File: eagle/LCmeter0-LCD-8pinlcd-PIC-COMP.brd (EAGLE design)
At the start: 58.4 x 50.8 mm, 34 parts, among them IC1 PIC16F876A-X/SP, J1 HD44780-4BIT-8PIN, J2 PIC-UART, J3 PIC-ICSP, K2 DS2Y, Q1 20MHz, T1 BC547CBE-A, X1 FREQ, X2 L/C

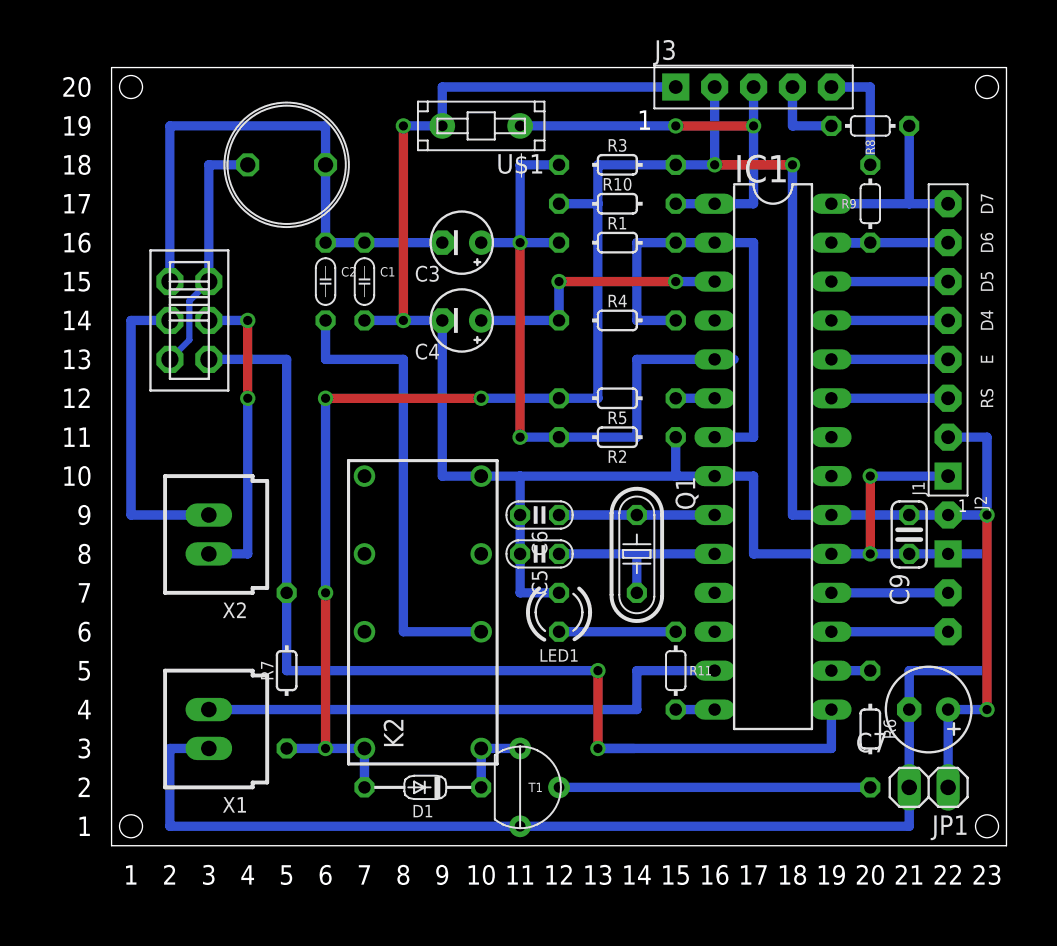
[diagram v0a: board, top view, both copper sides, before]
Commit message: ...
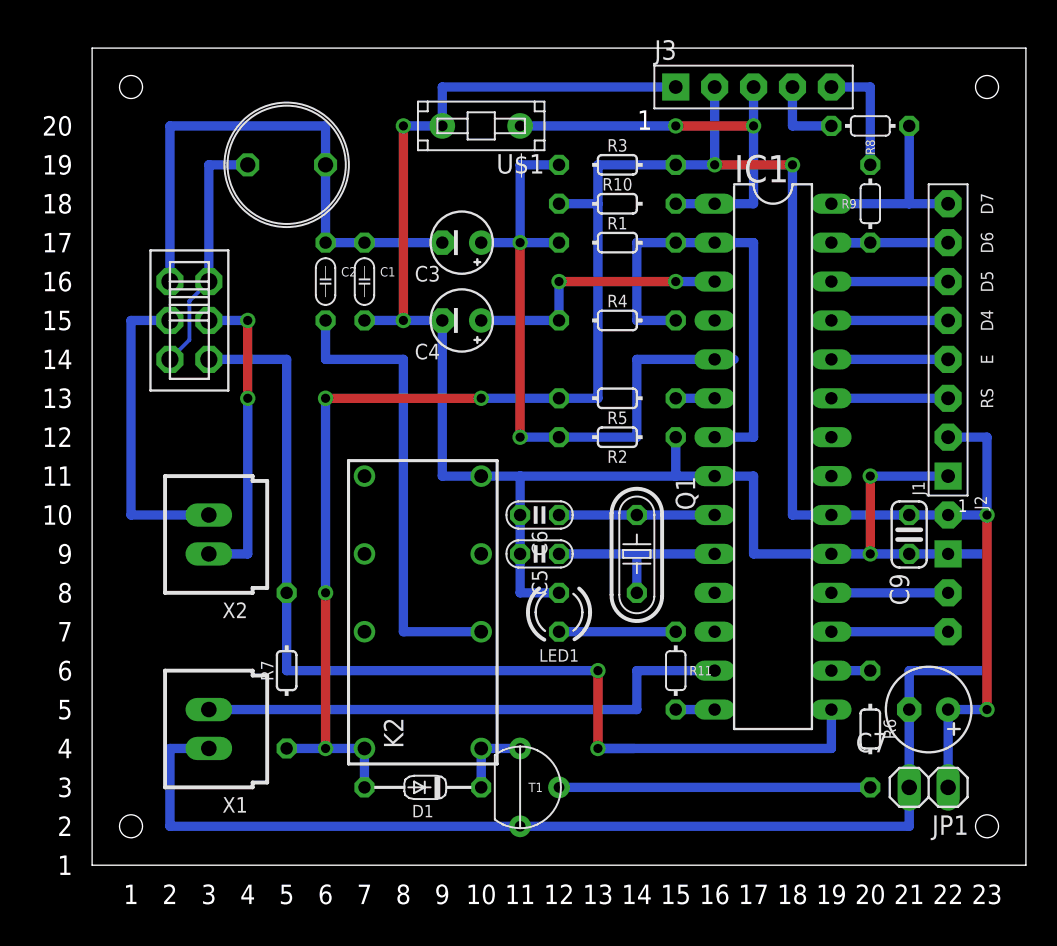
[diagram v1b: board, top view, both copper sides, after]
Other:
- board size 58.4 x 50.8 mm -> 61 x 53.3 mm
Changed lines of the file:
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@@
 <board>
 <plain>
-<wire x1="-1.27" y1="-1.27" x2="57.15" y2="-1.27" width="0" layer="20"/>
-<wire x1="57.15" y1="-1.27" x2="57.15" y2="49.53" width="0" layer="20"/>
-<wire x1="57.15" y1="49.53" x2="-1.27" y2="49.53" width="0" layer="20"/>
-<wire x1="-1.27" y1="49.53" x2="-1.27" y2="-1.27" width="0" layer="20"/>
+<wire x1="-2.54" y1="-2.54" x2="58.42" y2="-2.54" width="0" layer="20"/>
+<wire x1="58.42" y1="-2.54" x2="58.42" y2="50.8" width="0" layer="20"/>
+<wire x1="58.42" y1="50.8" x2="-2.54" y2="50.8" width="0" layer="20"/>
+<wire x1="-2.54" y1="50.8" x2="-2.54" y2="-2.54" width="0" layer="20"/>
 <text x="55.88" y="40.64" size="0.8128" layer="21" rot="R90" align="center">D7</text>
 <text x="55.88" y="38.1" size="0.8128" layer="21" rot="R90" align="center">D6</text>
@@
 <text x="55.88" y="30.48" size="0.8128" layer="21" rot="R90" align="center">E</text>
 <text x="55.88" y="27.94" size="0.8128" layer="21" rot="R90" align="center">RS</text>
-<text x="-2.54" y="0" size="1.27" layer="20" align="center-right">1</text>
-<text x="-2.54" y="2.54" size="1.27" layer="20" align="center-right">2</text>
-<text x="-2.54" y="5.08" size="1.27" layer="20" align="center-right">3</text>
-<text x="-2.54" y="7.62" size="1.27" layer="20" align="center-right">4</text>
-<text x="-2.54" y="10.16" size="1.27" layer="20" align="center-right">5</text>
-<text x="-2.54" y="12.7" size="1.27" layer="20" align="center-right">6</text>
-<text x="-2.54" y="15.24" size="1.27" layer="20" align="center-right">7</text>
-<text x="-2.54" y="17.78" size="1.27" layer="20" align="center-right">8</text>
-<text x="-2.54" y="20.32" size="1.27" layer="20" align="center-right">9</text>
-<text x="-2.54" y="22.86" size="1.27" layer="20" align="center-right">10</text>
-<text x="-2.54" y="25.4" size="1.27" layer="20" align="center-right">11</text>
-<text x="-2.54" y="27.94" size="1.27" layer="20" align="center-right">12</text>
-<text x="-2.54" y="30.48" size="1.27" layer="20" align="center-right">13</text>
-<text x="-2.54" y="33.02" size="1.27" layer="20" align="center-right">14</text>
-<text x="-2.54" y="35.56" size="1.27" layer="20" align="center-right">15</text>
-<text x="-2.54" y="38.1" size="1.27" layer="20" align="center-right">16</text>
-<text x="-2.54" y="40.64" size="1.27" layer="20" align="center-right">17</text>
-<text x="-2.54" y="43.18" size="1.27" layer="20" align="center-right">18</text>
-<text x="-2.54" y="45.72" size="1.27" layer="20" align="center-right">19</text>
-<text x="-2.54" y="48.26" size="1.27" layer="20" align="center-right">20</text>
-<text x="0" y="-2.54" size="1.27" layer="20" align="top-center">1</text>
-<text x="2.54" y="-2.54" size="1.27" layer="20" align="top-center">2</text>
-<text x="5.08" y="-2.54" size="1.27" layer="20" align="top-center">3</text>
-<text x="7.62" y="-2.54" size="1.27" layer="20" align="top-center">4</text>
-<text x="10.16" y="-2.54" size="1.27" layer="20" align="top-center">5</text>
-<text x="12.7" y="-2.54" size="1.27" layer="20" align="top-center">6</text>
-<text x="15.24" y="-2.54" size="1.27" layer="20" align="top-center">7</text>
-<text x="17.78" y="-2.54" size="1.27" layer="20" align="top-center">8</text>
-<text x="20.32" y="-2.54" size="1.27" layer="20" align="top-center">9</text>
-<text x="22.86" y="-2.54" size="1.27" layer="20" align="top-center">10</text>
-<text x="25.4" y="-2.54" size="1.27" layer="20" align="top-center">11</text>
-<text x="27.94" y="-2.54" size="1.27" layer="20" align="top-center">12</text>
-<text x="30.48" y="-2.54" size="1.27" layer="20" align="top-center">13</text>
-<text x="33.02" y="-2.54" size="1.27" layer="20" align="top-center">14</text>
-<text x="35.56" y="-2.54" size="1.27" layer="20" align="top-center">15</text>
-<text x="38.1" y="-2.54" size="1.27" layer="20" align="top-center">16</text>
-<text x="40.64" y="-2.54" size="1.27" layer="20" align="top-center">17</text>
-<text x="43.18" y="-2.54" size="1.27" layer="20" align="top-center">18</text>
-<text x="45.72" y="-2.54" size="1.27" layer="20" align="top-center">19</text>
-<text x="48.26" y="-2.54" size="1.27" layer="20" align="top-center">20</text>
-<text x="50.8" y="-2.54" size="1.27" layer="20" align="top-center">21</text>
-<text x="53.34" y="-2.54" size="1.27" layer="20" align="top-center">22</text>
-<text x="55.88" y="-2.54" size="1.27" layer="20" align="top-center">23</text>
+<text x="-3.81" y="-2.54" size="1.27" layer="20" align="center-right">1</text>
+<text x="-3.81" y="0" size="1.27" layer="20" align="center-right">2</text>
+<text x="-3.81" y="2.54" size="1.27" layer="20" align="center-right">3</text>
+<text x="-3.81" y="5.08" size="1.27" layer="20" align="center-right">4</text>
+<text x="-3.81" y="7.62" size="1.27" layer="20" align="center-right">5</text>
+<text x="-3.81" y="10.16" size="1.27" layer="20" align="center-right">6</text>
+<text x="-3.81" y="12.7" size="1.27" layer="20" align="center-right">7</text>
+<text x="-3.81" y="15.24" size="1.27" layer="20" align="center-right">8</text>
+<text x="-3.81" y="17.78" size="1.27" layer="20" align="center-right">9</text>
+<text x="-3.81" y="20.32" size="1.27" layer="20" align="center-right">10</text>
+<text x="-3.81" y="22.86" size="1.27" layer="20" align="center-right">11</text>
+<text x="-3.81" y="25.4" size="1.27" layer="20" align="center-right">12</text>
+<text x="-3.81" y="27.94" size="1.27" layer="20" align="center-right">13</text>
+<text x="-3.81" y="30.48" size="1.27" layer="20" align="center-right">14</text>
+<text x="-3.81" y="33.02" size="1.27" layer="20" align="center-right">15</text>
+<text x="-3.81" y="35.56" size="1.27" layer="20" align="center-right">16</text>
+<text x="-3.81" y="38.1" size="1.27" layer="20" align="center-right">17</text>
+<text x="-3.81" y="40.64" size="1.27" layer="20" align="center-right">18</text>
+<text x="-3.81" y="43.18" size="1.27" layer="20" align="center-right">19</text>
+<text x="-3.81" y="45.72" size="1.27" layer="20" align="center-right">20</text>
+<text x="0" y="-3.81" size="1.27" layer="20" align="top-center">1</text>
+<text x="2.54" y="-3.81" size="1.27" layer="20" align="top-center">2</text>
+<text x="5.08" y="-3.81" size="1.27" layer="20" align="top-center">3</text>
+<text x="7.62" y="-3.81" size="1.27" layer="20" align="top-center">4</text>
+<text x="10.16" y="-3.81" size="1.27" layer="20" align="top-center">5</text>
+<text x="12.7" y="-3.81" size="1.27" layer="20" align="top-center">6</text>
+<text x="15.24" y="-3.81" size="1.27" layer="20" align="top-center">7</text>
+<text x="17.78" y="-3.81" size="1.27" layer="20" align="top-center">8</text>
+<text x="20.32" y="-3.81" size="1.27" layer="20" align="top-center">9</text>
+<text x="22.86" y="-3.81" size="1.27" layer="20" align="top-center">10</text>
+<text x="25.4" y="-3.81" size="1.27" layer="20" align="top-center">11</text>
+<text x="27.94" y="-3.81" size="1.27" layer="20" align="top-center">12</text>
+<text x="30.48" y="-3.81" size="1.27" layer="20" align="top-center">13</text>
+<text x="33.02" y="-3.81" size="1.27" layer="20" align="top-center">14</text>
+<text x="35.56" y="-3.81" size="1.27" layer="20" align="top-center">15</text>
+<text x="38.1" y="-3.81" size="1.27" layer="20" align="top-center">16</text>
+<text x="40.64" y="-3.81" size="1.27" layer="20" align="top-center">17</text>
+<text x="43.18" y="-3.81" size="1.27" layer="20" align="top-center">18</text>
+<text x="45.72" y="-3.81" size="1.27" layer="20" align="top-center">19</text>
+<text x="48.26" y="-3.81" size="1.27" layer="20" align="top-center">20</text>
+<text x="50.8" y="-3.81" size="1.27" layer="20" align="top-center">21</text>
+<text x="53.34" y="-3.81" size="1.27" layer="20" align="top-center">22</text>
+<text x="55.88" y="-3.81" size="1.27" layer="20" align="top-center">23</text>
 <hole x="0" y="48.26" drill="1.5"/>
 <hole x="55.88" y="48.26" drill="1.5"/>
@@
 <wire x1="5.08" y1="35.56" x2="5.08" y2="43.18" width="0.6096" layer="16"/>
 <wire x1="5.08" y1="43.18" x2="7.62" y2="43.18" width="0.6096" layer="16"/>
-<wire x1="5.08" y1="35.56" x2="3.81" y2="34.29" width="0.4064" layer="16"/>
-<wire x1="3.81" y1="34.29" x2="3.81" y2="31.75" width="0.4064" layer="16"/>
-<wire x1="3.81" y1="31.75" x2="2.54" y2="30.48" width="0.4064" layer="16"/>
+<wire x1="5.08" y1="35.56" x2="3.81" y2="34.29" width="0.254" layer="16"/>
+<wire x1="3.81" y1="34.29" x2="3.81" y2="31.75" width="0.254" layer="16"/>
+<wire x1="3.81" y1="31.75" x2="2.54" y2="30.48" width="0.254" layer="16"/>
 </signal>
 <signal name="OSC1">

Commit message: ...
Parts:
- L1: value 100μH -> 68μH
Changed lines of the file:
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@@
 <element name="D1" library="d" package="DO34-7" value="1N4148" x="19.05" y="2.54" rot="R180"/>
 <element name="IC1" library="lc-meter" package="DIL28-3" value="PIC16F876A-X/SP" x="41.91" y="24.13" rot="R270"/>
-<element name="L1" library="r" package="L-09R" value="100μH" x="10.16" y="43.18"/>
+<element name="L1" library="r" package="L-09R" value="68μH" x="10.16" y="43.18"/>
 <element name="Q1" library="q" package="HC49" value="20MHz" x="33.02" y="17.78" rot="R270"/>
 <element name="R1" library="r" package="0202/7" value="100kΩ" x="31.75" y="38.1" rot="R270"/>
